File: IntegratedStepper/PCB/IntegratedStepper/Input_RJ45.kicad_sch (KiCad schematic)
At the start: 6 parts, among them J1 8P8C, J2 8P8C, J5 Conn_01x05_Socket, P1 USB_C_Plug

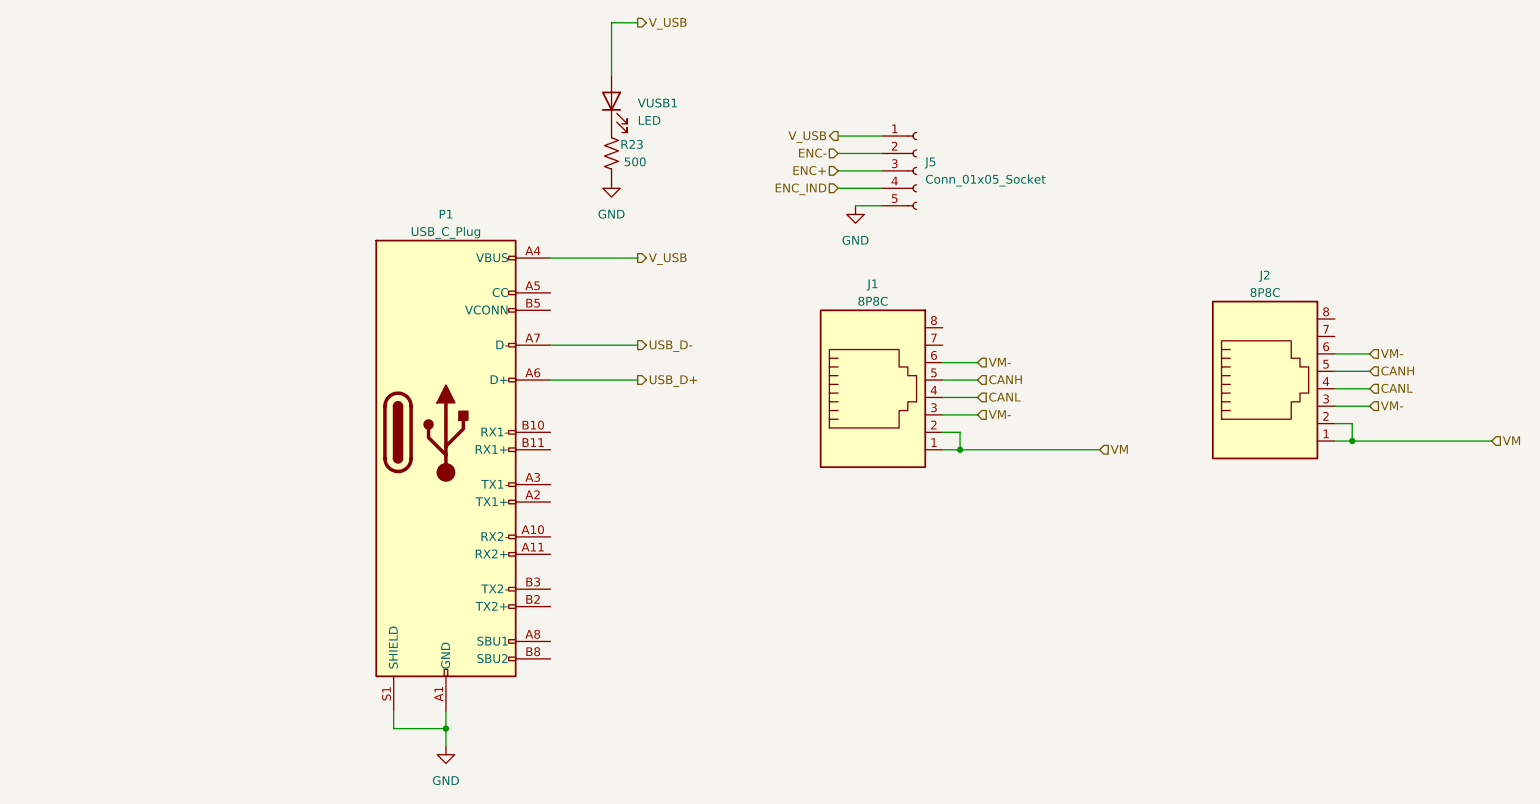
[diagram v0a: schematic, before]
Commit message: Add final layout + 3D models
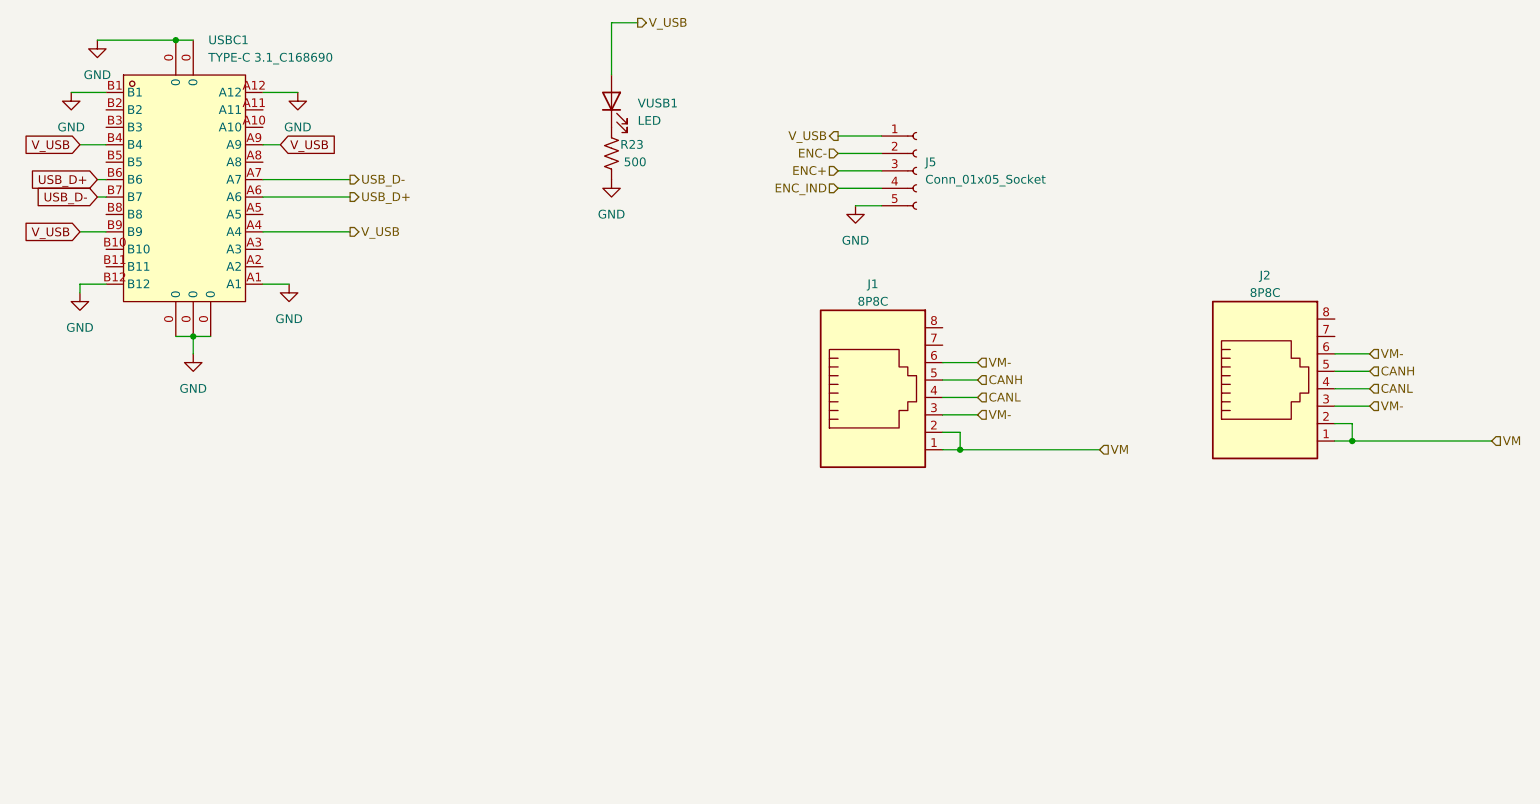
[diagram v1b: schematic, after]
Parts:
- removed P1: USB_C_Plug, Connector_USB:USB_C_Receptacle_G-Switch_GT-USB-7051x, symbol Connector:USB_C_Plug
- added USBC1: TYPE-C 3.1_C168690, easyeda2kicad:USB-C-SMD_TYPE-C-USB-3, symbol easyeda2kicad:TYPE-C3.1_C168690
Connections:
- net GND: now also USBC1.0, USBC1.A1, USBC1.A12, USBC1.B1, USBC1.B12
- net USB_D+: now also USBC1.A6, USBC1.B6
- net USB_D-: now also USBC1.A7, USBC1.B7
- net V_USB: now also USBC1.A4, USBC1.A9, USBC1.B4, USBC1.B9
